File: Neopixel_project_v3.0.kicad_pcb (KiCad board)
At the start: 2 copper layers, 50 x 50 mm, 64 parts, among them J1 Conn_01x03_Pin, J3 Screw_Terminal_01x02, Q1 MMBT3904, Q2 MMBT3904, Q3 MMBT3904, Q4 MMBT3904, Q5 DO3407B, Q6 DO3407B, Q7 DO3407B, Q8 DO3407B, SW1 TS-1088-AR02016, SW2 TS-1088-AR02016, U1 ESP8685H4, U2 AL8843, U3 TD1469, U4 USBLC6-4SC6, Y1 Crystal_GND24

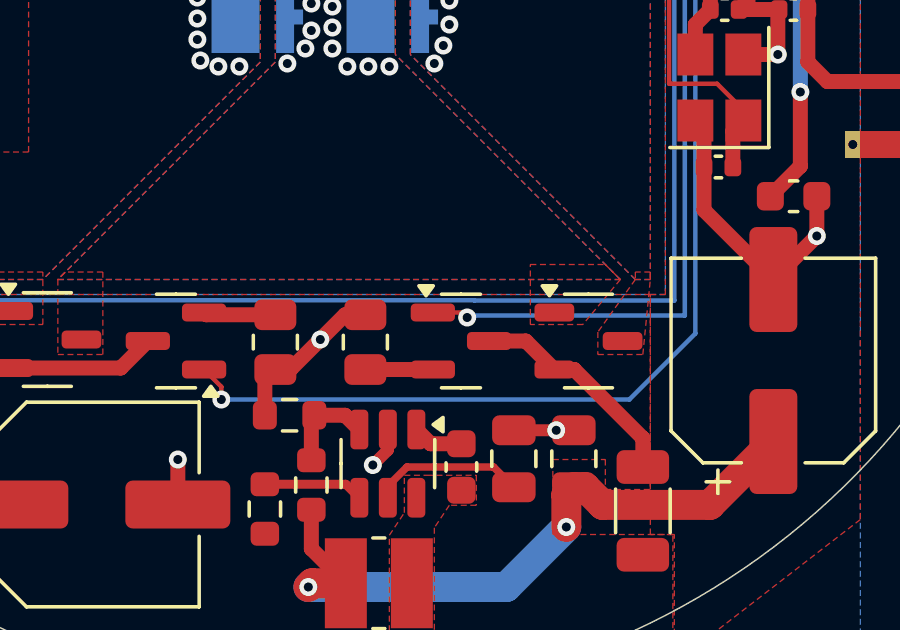
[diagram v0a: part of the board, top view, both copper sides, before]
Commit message: added gerber files
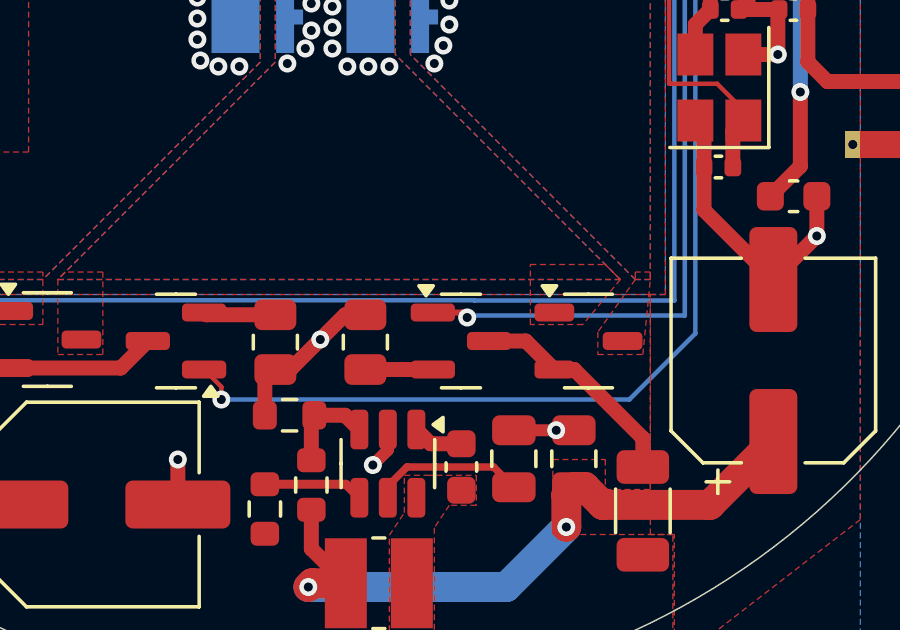
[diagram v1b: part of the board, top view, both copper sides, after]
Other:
- rule pad_to_mask_clearance: 0.05 -> 0
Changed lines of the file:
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@@
 			(dielectric_constraints no)
 		)
-		(pad_to_mask_clearance 0.05)
+		(pad_to_mask_clearance 0)
 		(allow_soldermask_bridges_in_footprints no)
 		(pcbplotparams
@@
 			(outputformat 1)
 			(mirror no)
-			(drillshape 1)
+			(drillshape 0)
 			(scaleselection 1)
-			(outputdirectory "")
+			(outputdirectory "gerber/")
 		)
 	)
@@
 	)
 	(segment
+		(start 108.578339 79.2)
+		(end 108.744124 79.365785)
+		(width 0.2)
+		(layer "F.Cu")
+		(net 30)
+	)
+	(segment
 		(start 117.45 58.6)
 		(end 117.45 58.966116)
@@
 	)
 	(segment
-		(start 108.578339 79.2)
-		(end 107.6 79.2)
-		(width 0.15)
+		(start 107.6 79.2)
+		(end 108.578339 79.2)
+		(width 0.2)
 		(layer "F.Cu")
 		(net 30)
@@
 		(width 0.15)
 		(layer "F.Cu")
-		(net 30)
-	)
-	(segment
-		(start 108.744124 79.365785)
-		(end 108.578339 79.2)
-		(width 0.15)
-		(layer "F.Cu")
